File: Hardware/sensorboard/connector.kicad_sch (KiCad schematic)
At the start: 0 parts

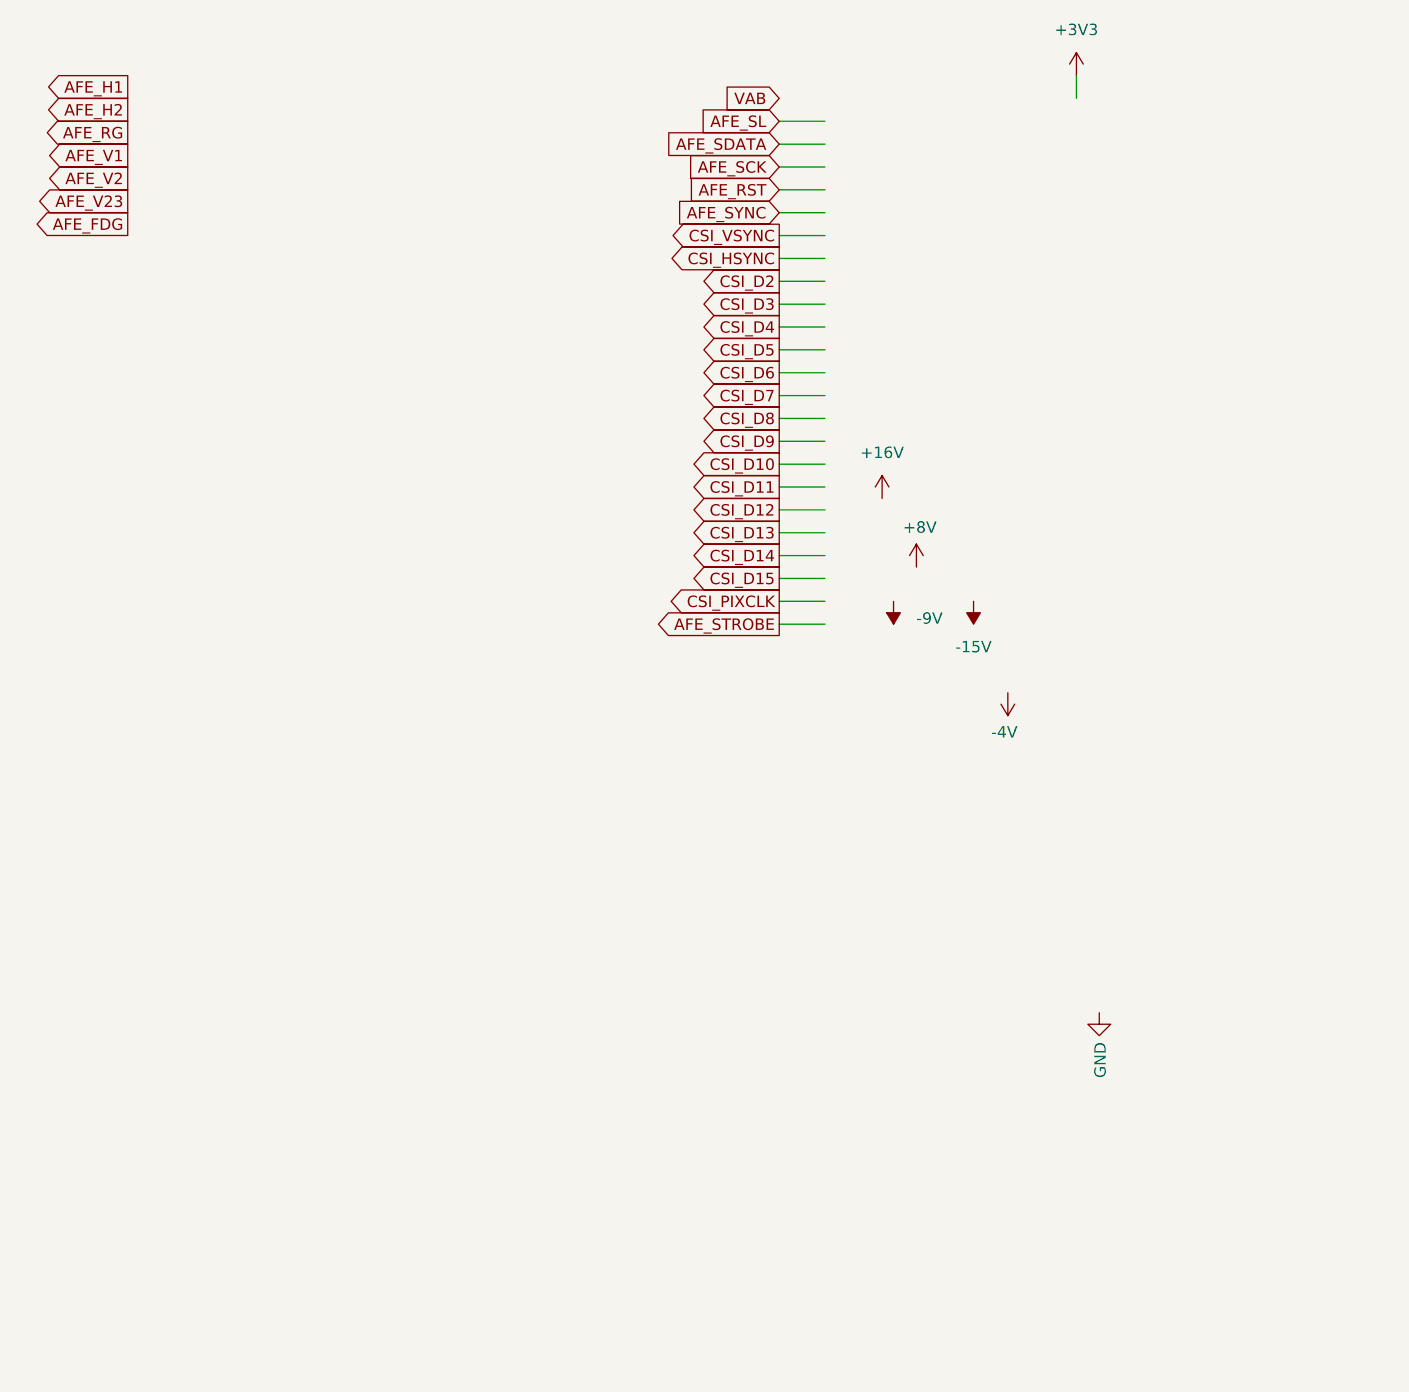
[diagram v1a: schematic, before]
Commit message: Update sensor/power board outline
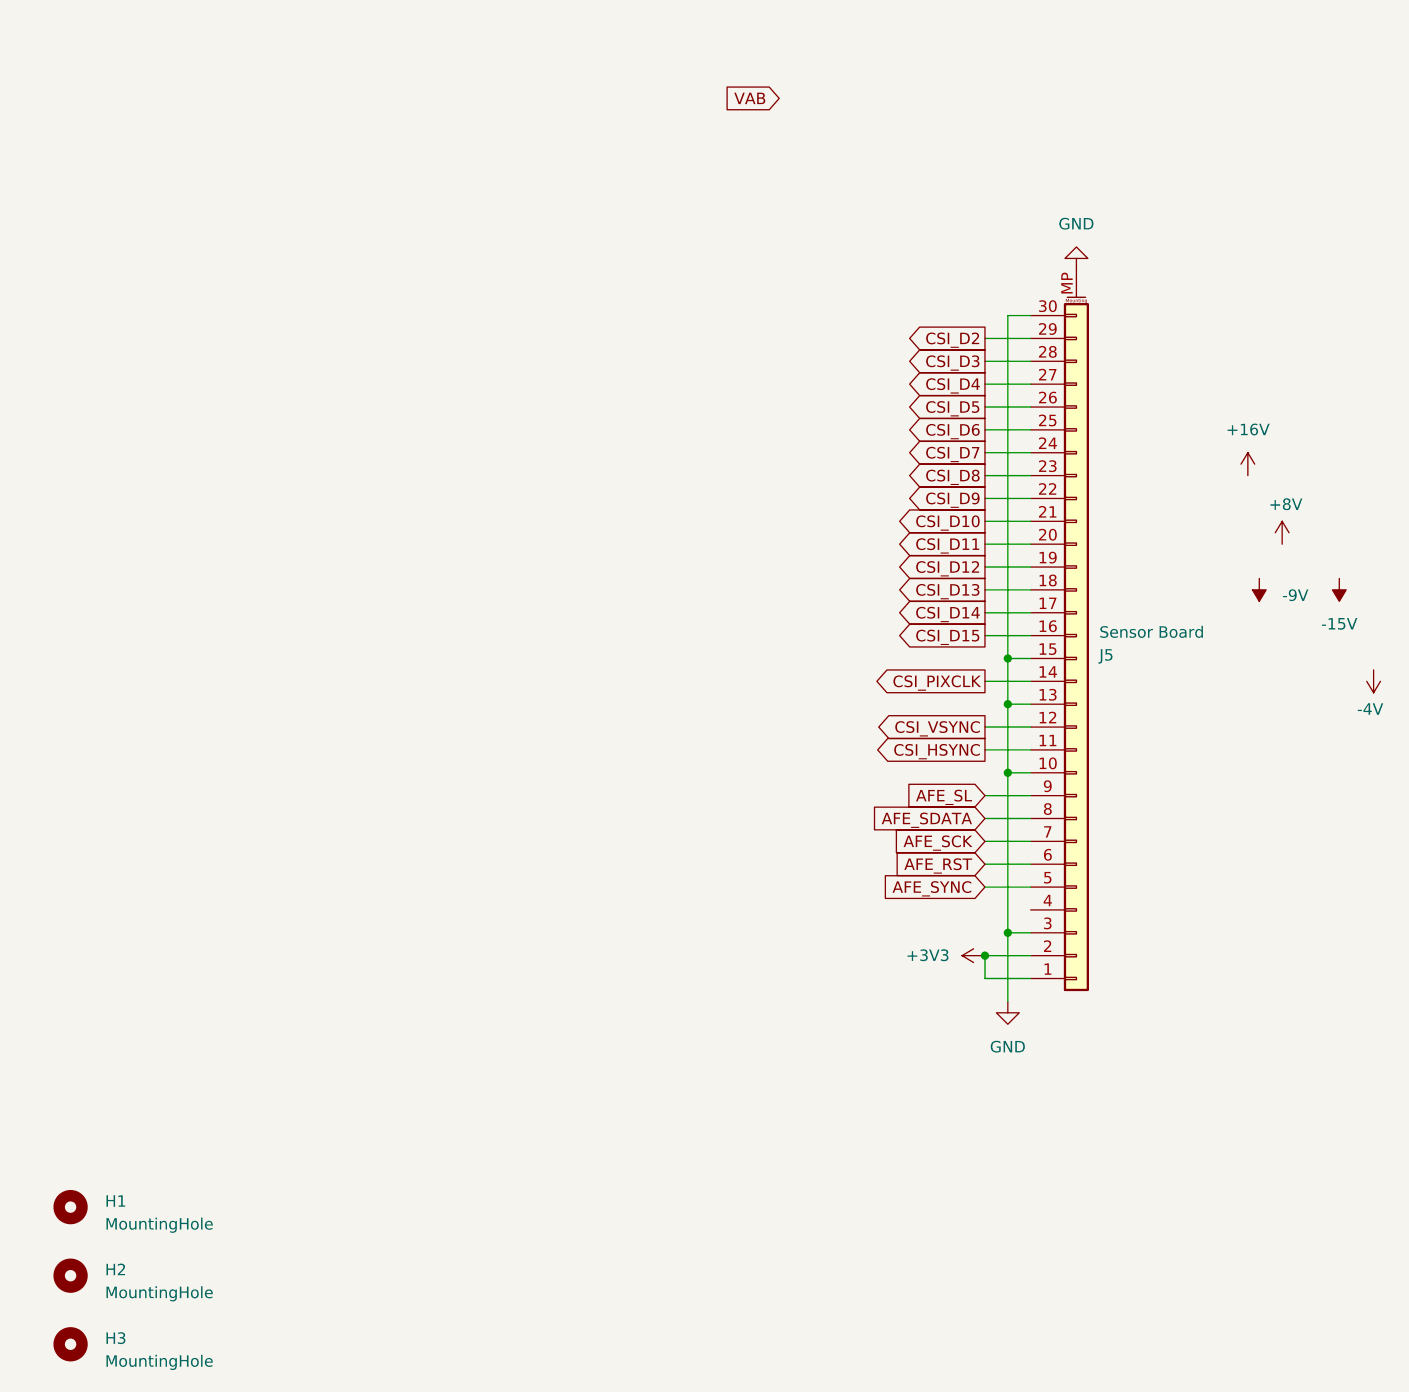
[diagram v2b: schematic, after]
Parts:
- added H1, H2, H3: MountingHole, MountingHole:MountingHole_2.2mm_M2_DIN965, symbol Mechanical:MountingHole
- added J5: Sensor Board, Connector_FFC-FPC:Hirose_FH12-30S-0.5SH_1x30-1MP_P0.50mm_Horizontal, symbol Connector_Generic_MountingPin:Conn_01x30_MountingPin
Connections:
- net +3V3: now also J5.1 (Pin_1), J5.2 (Pin_2)
- net AFE_RST: now also J5.6 (Pin_6)
- net AFE_SCK: now also J5.7 (Pin_7)
- net AFE_SDATA: now also J5.8 (Pin_8)
- net AFE_SL: now also J5.9 (Pin_9)
- net AFE_SYNC: now also J5.5 (Pin_5)
- net CSI_D10: now also J5.21 (Pin_21)
- net CSI_D11: now also J5.20 (Pin_20)
- net CSI_D12: now also J5.19 (Pin_19)
- net CSI_D13: now also J5.18 (Pin_18)
- net CSI_D14: now also J5.17 (Pin_17)
- net CSI_D15: now also J5.16 (Pin_16)
- net CSI_D2: now also J5.29 (Pin_29)
- net CSI_D3: now also J5.28 (Pin_28)
- net CSI_D4: now also J5.27 (Pin_27)
- net CSI_D5: now also J5.26 (Pin_26)
- net CSI_D6: now also J5.25 (Pin_25)
- net CSI_D7: now also J5.24 (Pin_24)
- net CSI_D8: now also J5.23 (Pin_23)
- net CSI_D9: now also J5.22 (Pin_22)
- net CSI_HSYNC: now also J5.11 (Pin_11)
- net CSI_PIXCLK: now also J5.14 (Pin_14)
- net CSI_VSYNC: now also J5.12 (Pin_12)
- net GND: now also J5.10 (Pin_10), J5.13 (Pin_13), J5.15 (Pin_15), J5.3 (Pin_3), J5.30 (Pin_30), J5.MP (MountPin)
